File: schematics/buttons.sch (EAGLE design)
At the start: 10 parts

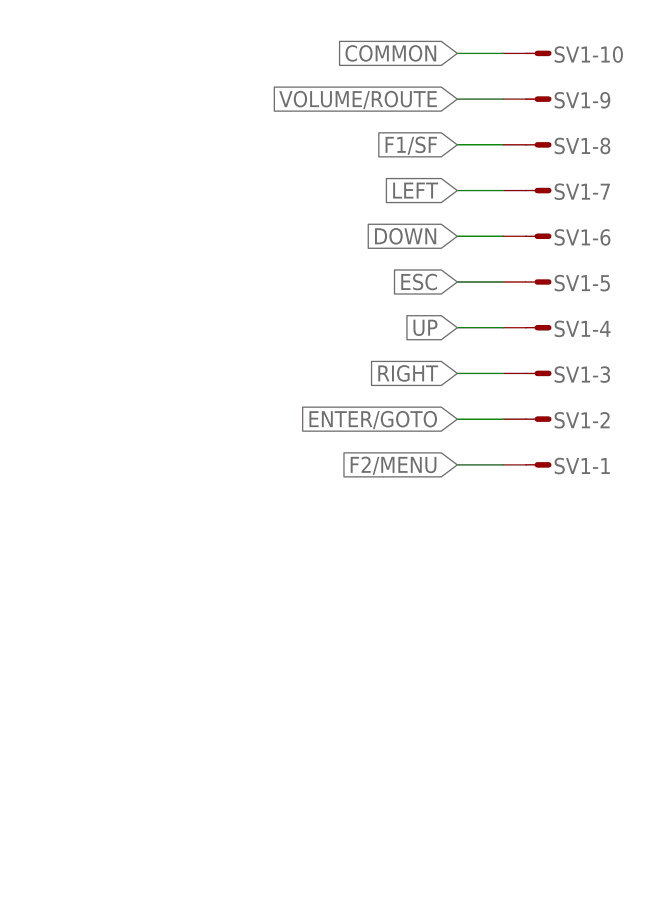
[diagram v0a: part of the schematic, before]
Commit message: Added screenshot for buttons
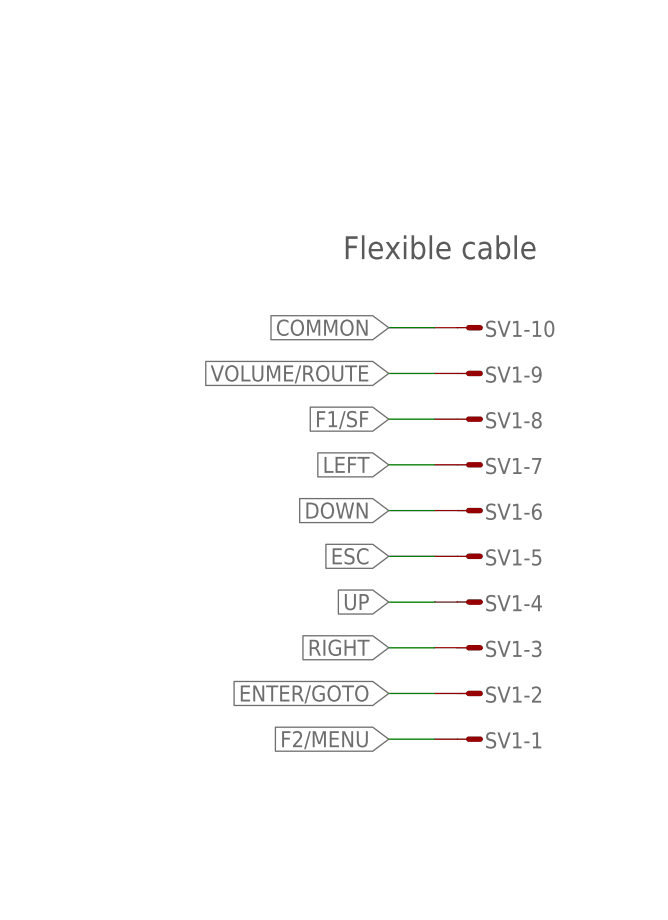
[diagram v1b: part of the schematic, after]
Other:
- note added: "Flexible cable"
- moved on the sheet: SV1-1, SV1-10, SV1-2, SV1-3, SV1-4, SV1-5, SV1-6, SV1-7, SV1-8, SV1-9
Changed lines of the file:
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@@
 <sheet>
 <plain>
+<frame x1="-22.86" y1="-45.72" x2="132.08" y2="83.82" columns="8" rows="5" layer="97"/>
+<text x="91.44" y="48.26" size="2.54" layer="97">Flexible cable</text>
 </plain>
 <instances>
@@
 <attribute name="VALUE" x="18.415" y="-31.75" size="1.778" layer="96"/>
 </instance>
-<instance part="SV1" gate="-1" x="114.3" y="25.4" smashed="yes" rot="R180">
-<attribute name="NAME" x="114.808" y="24.384" size="1.778" layer="95"/>
-<attribute name="VALUE" x="114.046" y="27.813" size="1.778" layer="96" rot="R180"/>
-</instance>
-<instance part="SV1" gate="-2" x="114.3" y="30.48" smashed="yes" rot="R180">
-<attribute name="NAME" x="114.808" y="29.464" size="1.778" layer="95"/>
-<attribute name="VALUE" x="114.046" y="32.893" size="1.778" layer="96" rot="R180"/>
-</instance>
-<instance part="SV1" gate="-3" x="114.3" y="35.56" smashed="yes" rot="R180">
-<attribute name="NAME" x="114.808" y="34.544" size="1.778" layer="95"/>
-<attribute name="VALUE" x="114.046" y="37.973" size="1.778" layer="96" rot="R180"/>
-</instance>
-<instance part="SV1" gate="-4" x="114.3" y="40.64" smashed="yes" rot="R180">
-<attribute name="NAME" x="114.808" y="39.624" size="1.778" layer="95"/>
-<attribute name="VALUE" x="114.046" y="43.053" size="1.778" layer="96" rot="R180"/>
-</instance>
-<instance part="SV1" gate="-5" x="114.3" y="45.72" smashed="yes" rot="R180">
-<attribute name="NAME" x="114.808" y="44.704" size="1.778" layer="95"/>
-<attribute name="VALUE" x="114.046" y="48.133" size="1.778" layer="96" rot="R180"/>
-</instance>
-<instance part="SV1" gate="-6" x="114.3" y="50.8" smashed="yes" rot="R180">
-<attribute name="NAME" x="114.808" y="49.784" size="1.778" layer="95"/>
-<attribute name="VALUE" x="114.046" y="53.213" size="1.778" layer="96" rot="R180"/>
-</instance>
-<instance part="SV1" gate="-7" x="114.3" y="55.88" smashed="yes" rot="R180">
-<attribute name="NAME" x="114.808" y="54.864" size="1.778" layer="95"/>
-<attribute name="VALUE" x="114.046" y="58.293" size="1.778" layer="96" rot="R180"/>
-</instance>
-<instance part="SV1" gate="-8" x="114.3" y="60.96" smashed="yes" rot="R180">
-<attribute name="NAME" x="114.808" y="59.944" size="1.778" layer="95"/>
-<attribute name="VALUE" x="114.046" y="63.373" size="1.778" layer="96" rot="R180"/>
-</instance>
-<instance part="SV1" gate="-9" x="114.3" y="66.04" smashed="yes" rot="R180">
-<attribute name="NAME" x="114.808" y="65.024" size="1.778" layer="95"/>
-<attribute name="VALUE" x="114.046" y="68.453" size="1.778" layer="96" rot="R180"/>
-</instance>
-<instance part="SV1" gate="-10" x="114.3" y="71.12" smashed="yes" rot="R180">
-<attribute name="NAME" x="114.808" y="70.104" size="1.778" layer="95"/>
-<attribute name="VALUE" x="114.046" y="73.533" size="1.778" layer="96" rot="R180"/>
+<instance part="SV1" gate="-1" x="106.68" y="-5.08" smashed="yes" rot="R180">
+<attribute name="NAME" x="107.188" y="-6.096" size="1.778" layer="95"/>
+<attribute name="VALUE" x="106.426" y="-2.667" size="1.778" layer="96" rot="R180"/>
+</instance>
+<instance part="SV1" gate="-2" x="106.68" y="0" smashed="yes" rot="R180">
+<attribute name="NAME" x="107.188" y="-1.016" size="1.778" layer="95"/>
+<attribute name="VALUE" x="106.426" y="2.413" size="1.778" layer="96" rot="R180"/>
+</instance>
+<instance part="SV1" gate="-3" x="106.68" y="5.08" smashed="yes" rot="R180">
+<attribute name="NAME" x="107.188" y="4.064" size="1.778" layer="95"/>
+<attribute name="VALUE" x="106.426" y="7.493" size="1.778" layer="96" rot="R180"/>
+</instance>
+<instance part="SV1" gate="-4" x="106.68" y="10.16" smashed="yes" rot="R180">
+<attribute name="NAME" x="107.188" y="9.144" size="1.778" layer="95"/>
+<attribute name="VALUE" x="106.426" y="12.573" size="1.778" layer="96" rot="R180"/>
+</instance>
+<instance part="SV1" gate="-5" x="106.68" y="15.24" smashed="yes" rot="R180">
+<attribute name="NAME" x="107.188" y="14.224" size="1.778" layer="95"/>
+<attribute name="VALUE" x="106.426" y="17.653" size="1.778" layer="96" rot="R180"/>
+</instance>
+<instance part="SV1" gate="-6" x="106.68" y="20.32" smashed="yes" rot="R180">
+<attribute name="NAME" x="107.188" y="19.304" size="1.778" layer="95"/>
+<attribute name="VALUE" x="106.426" y="22.733" size="1.778" layer="96" rot="R180"/>
+</instance>
+<instance part="SV1" gate="-7" x="106.68" y="25.4" smashed="yes" rot="R180">
+<attribute name="NAME" x="107.188" y="24.384" size="1.778" layer="95"/>
+<attribute name="VALUE" x="106.426" y="27.813" size="1.778" layer="96" rot="R180"/>
+</instance>
+<instance part="SV1" gate="-8" x="106.68" y="30.48" smashed="yes" rot="R180">
+<attribute name="NAME" x="107.188" y="29.464" size="1.778" layer="95"/>
+<attribute name="VALUE" x="106.426" y="32.893" size="1.778" layer="96" rot="R180"/>
+</instance>
+<instance part="SV1" gate="-9" x="106.68" y="35.56" smashed="yes" rot="R180">
+<attribute name="NAME" x="107.188" y="34.544" size="1.778" layer="95"/>
+<attribute name="VALUE" x="106.426" y="37.973" size="1.778" layer="96" rot="R180"/>
+</instance>
+<instance part="SV1" gate="-10" x="106.68" y="40.64" smashed="yes" rot="R180">
+<attribute name="NAME" x="107.188" y="39.624" size="1.778" layer="95"/>
+<attribute name="VALUE" x="106.426" y="43.053" size="1.778" layer="96" rot="R180"/>
 </instance>
 </instances>
@@
 <segment>
 <pinref part="SV1" gate="-10" pin="S"/>
-<wire x1="109.22" y1="71.12" x2="104.14" y2="71.12" width="0.1524" layer="91"/>
-<label x="104.14" y="71.12" size="1.778" layer="95" rot="R180" xref="yes"/>
+<wire x1="101.6" y1="40.64" x2="96.52" y2="40.64" width="0.1524" layer="91"/>
+<label x="96.52" y="40.64" size="1.778" layer="95" rot="R180" xref="yes"/>
 </segment>
 </net>
@@
 <segment>
 <pinref part="SV1" gate="-8" pin="S"/>
-<wire x1="109.22" y1="60.96" x2="104.14" y2="60.96" width="0.1524" layer="91"/>
-<label x="104.14" y="60.96" size="1.778" layer="95" rot="R180" xref="yes"/>
+<wire x1="101.6" y1="30.48" x2="96.52" y2="30.48" width="0.1524" layer="91"/>
+<label x="96.52" y="30.48" size="1.778" layer="95" rot="R180" xref="yes"/>
 </segment>
 </net>
@@
 <segment>
 <pinref part="SV1" gate="-9" pin="S"/>
-<wire x1="109.22" y1="66.04" x2="104.14" y2="66.04" width="0.1524" layer="91"/>
-<label x="104.14" y="66.04" size="1.778" layer="95" rot="R180" xref="yes"/>
+<wire x1="101.6" y1="35.56" x2="96.52" y2="35.56" width="0.1524" layer="91"/>
+<label x="96.52" y="35.56" size="1.778" layer="95" rot="R180" xref="yes"/>
 </segment>
 </net>
@@
 <segment>
 <pinref part="SV1" gate="-5" pin="S"/>
-<wire x1="109.22" y1="45.72" x2="104.14" y2="45.72" width="0.1524" layer="91"/>
-<label x="104.14" y="45.72" size="1.778" layer="95" rot="R180" xref="yes"/>
+<wire x1="101.6" y1="15.24" x2="96.52" y2="15.24" width="0.1524" layer="91"/>
+<label x="96.52" y="15.24" size="1.778" layer="95" rot="R180" xref="yes"/>
 </segment>
 </net>
@@
 <segment>
 <pinref part="SV1" gate="-2" pin="S"/>
-<wire x1="109.22" y1="30.48" x2="104.14" y2="30.48" width="0.1524" layer="91"/>
-<label x="104.14" y="30.48" size="1.778" layer="95" rot="R180" xref="yes"/>
+<wire x1="101.6" y1="0" x2="96.52" y2="0" width="0.1524" layer="91"/>
+<label x="96.52" y="0" size="1.778" layer="95" rot="R180" xref="yes"/>
 </segment>
 </net>
@@
 <segment>
 <pinref part="SV1" gate="-1" pin="S"/>
-<wire x1="109.22" y1="25.4" x2="104.14" y2="25.4" width="0.1524" layer="91"/>
-<label x="104.14" y="25.4" size="1.778" layer="95" rot="R180" xref="yes"/>
+<wire x1="101.6" y1="-5.08" x2="96.52" y2="-5.08" width="0.1524" layer="91"/>
+<label x="96.52" y="-5.08" size="1.778" layer="95" rot="R180" xref="yes"/>
 </segment>
 </net>
@@
 <segment>
 <pinref part="SV1" gate="-4" pin="S"/>
-<wire x1="109.22" y1="40.64" x2="104.14" y2="40.64" width="0.1524" layer="91"/>
-<label x="104.14" y="40.64" size="1.778" layer="95" rot="R180" xref="yes"/>
+<wire x1="101.6" y1="10.16" x2="96.52" y2="10.16" width="0.1524" layer="91"/>
+<label x="96.52" y="10.16" size="1.778" layer="95" rot="R180" xref="yes"/>
 </segment>
 </net>
@@
 <segment>
 <pinref part="SV1" gate="-7" pin="S"/>
-<wire x1="109.22" y1="55.88" x2="104.14" y2="55.88" width="0.1524" layer="91"/>
-<label x="104.14" y="55.88" size="1.778" layer="95" rot="R180" xref="yes"/>
+<wire x1="101.6" y1="25.4" x2="96.52" y2="25.4" width="0.1524" layer="91"/>
+<label x="96.52" y="25.4" size="1.778" layer="95" rot="R180" xref="yes"/>
 </segment>
 </net>
@@
 <segment>
 <pinref part="SV1" gate="-6" pin="S"/>
-<wire x1="109.22" y1="50.8" x2="104.14" y2="50.8" width="0.1524" layer="91"/>
-<label x="104.14" y="50.8" size="1.778" layer="95" rot="R180" xref="yes"/>
+<wire x1="101.6" y1="20.32" x2="96.52" y2="20.32" width="0.1524" layer="91"/>
+<label x="96.52" y="20.32" size="1.778" layer="95" rot="R180" xref="yes"/>
 </segment>
 </net>
@@
 <segment>
 <pinref part="SV1" gate="-3" pin="S"/>
-<wire x1="109.22" y1="35.56" x2="104.14" y2="35.56" width="0.1524" layer="91"/>
-<label x="104.14" y="35.56" size="1.778" layer="95" rot="R180" xref="yes"/>
-</segment>
-</net>
+<wire x1="101.6" y1="5.08" x2="96.52" y2="5.08" width="0.1524" layer="91"/>
+<label x="96.52" y="5.08" size="1.778" layer="95" rot="R180" xref="yes"/>
+</segment>
+</net>
